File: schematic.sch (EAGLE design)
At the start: 25 parts

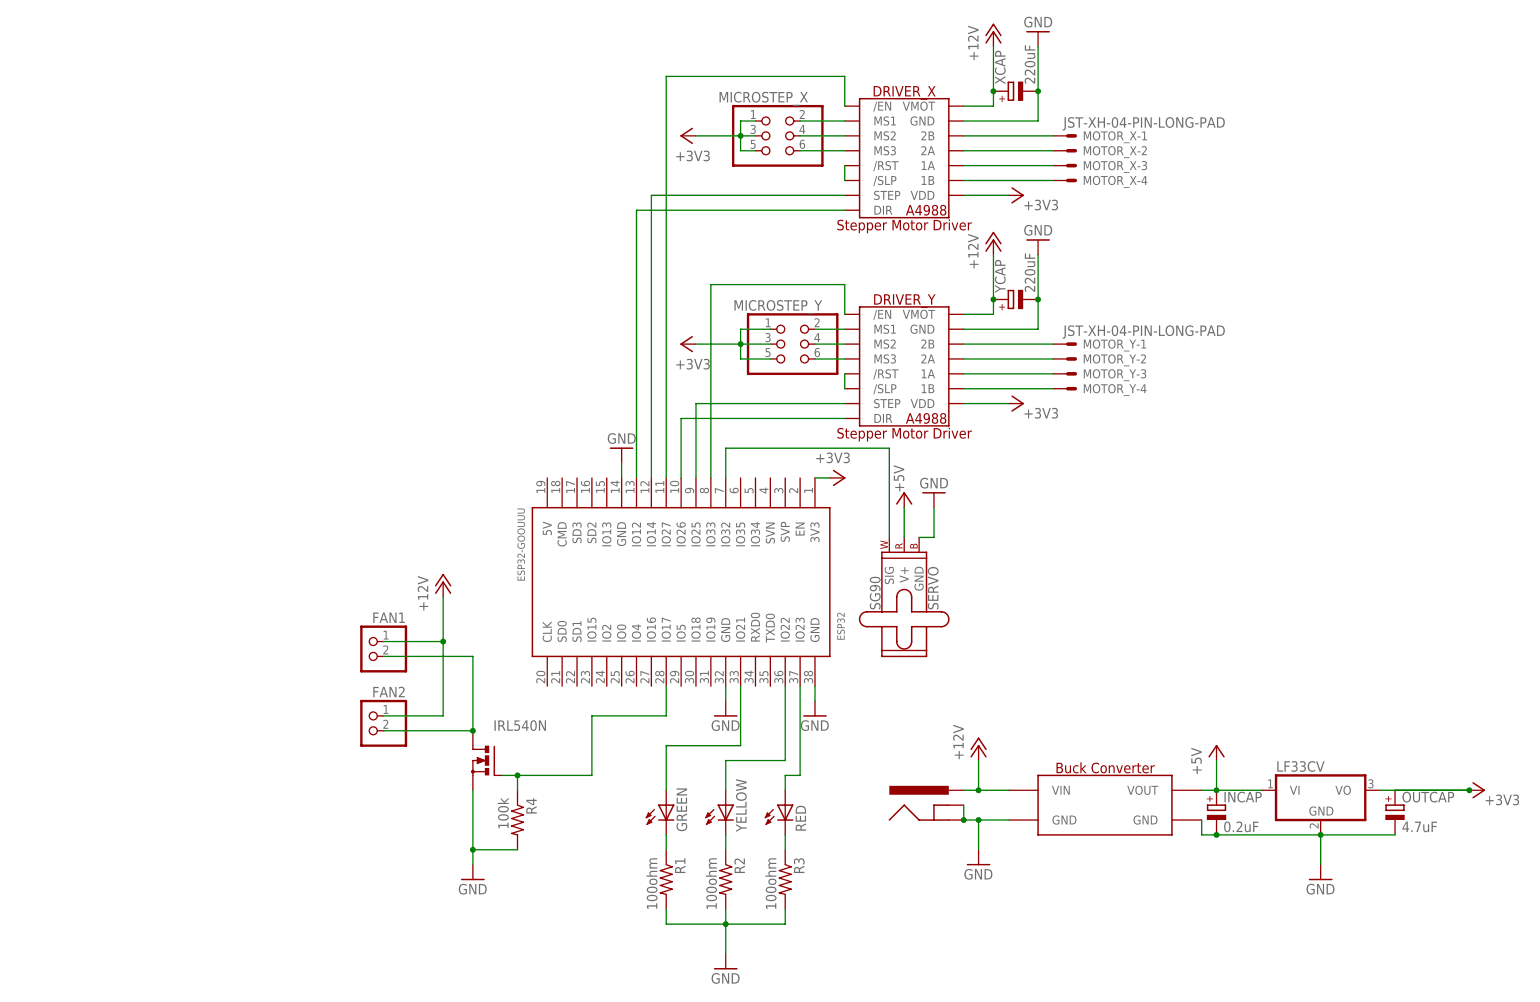
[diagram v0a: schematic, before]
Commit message: akjdf;sjf
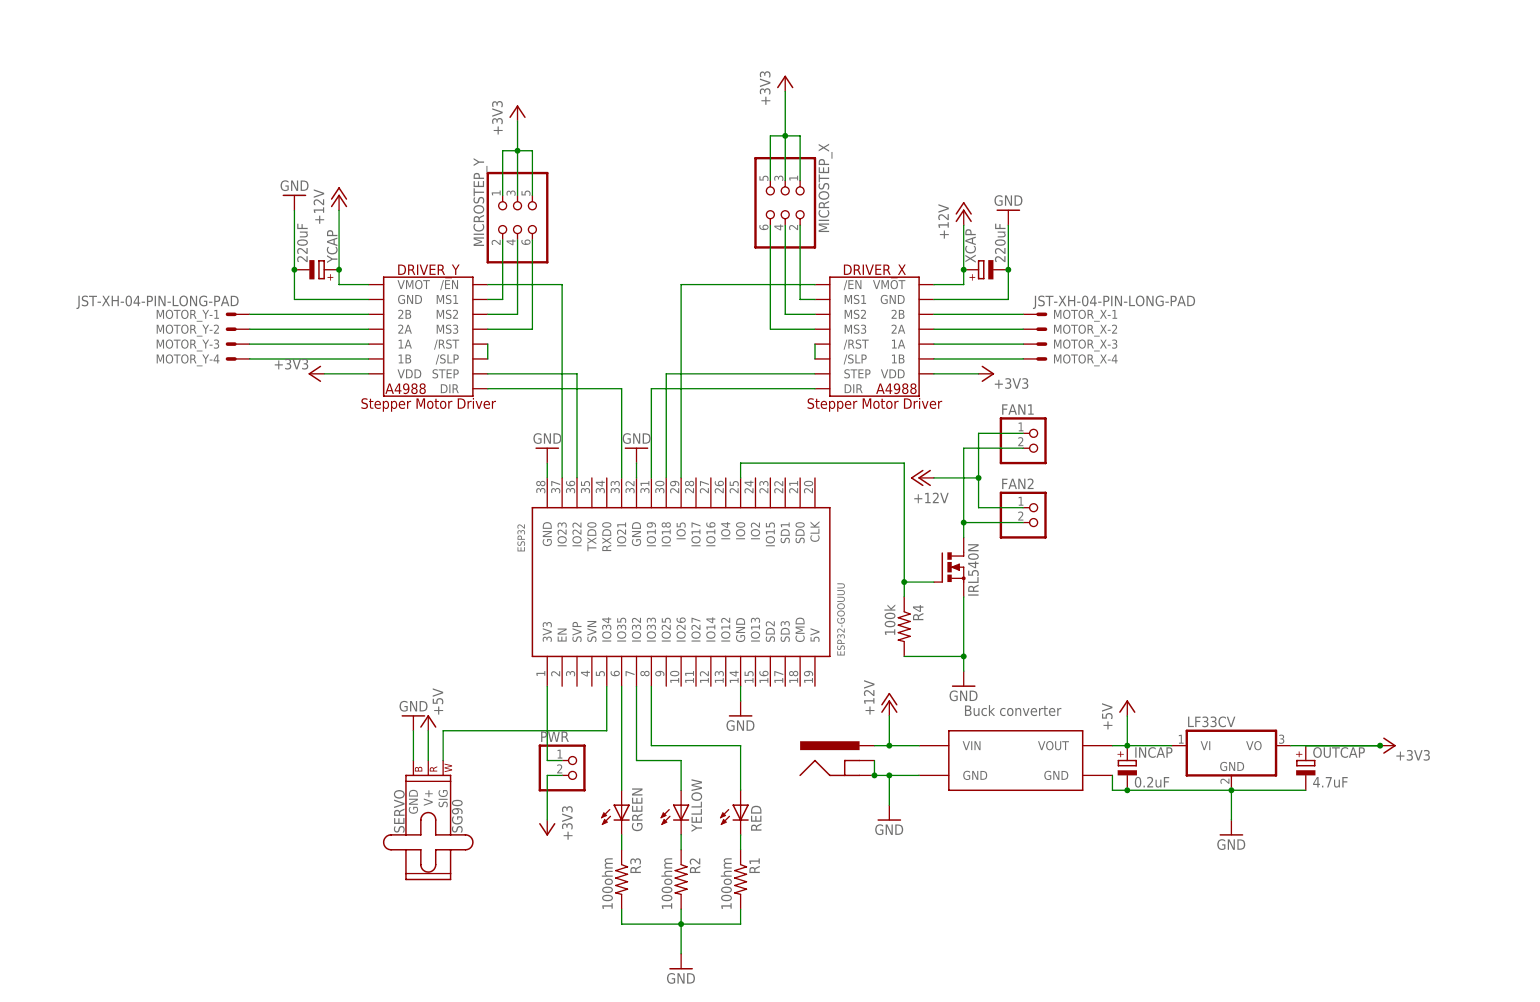
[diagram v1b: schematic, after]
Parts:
- removed U$1: BUCK-CONVERTER, buck-converter:BUCK-CONVERTER
- added PWR: (no value), pinhead:PINHD-1X2
- added U$2: BUCK-CONVERTER, mine:BUCK-CONVERTER
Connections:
- net MS1_X renamed N$11
- net MS1_Y renamed N$5
- net MS2_X renamed N$12
- net MS2_Y renamed N$9
- net MS3_X renamed N$13
- net MS3_Y renamed N$10
- net N$32 renamed FAN_PW
- removed net N$15: DRIVER_X./EN, ESP32.IO27
- removed net N$19: DRIVER_Y./EN, ESP32.IO33
- removed net N$2: DRIVER_X.STEP, ESP32.IO14
- removed net N$23: ESP32.IO23, RED.A
- removed net N$25: GREEN.C, R1.1
- removed net N$26: ESP32.IO21, GREEN.A
- removed net N$27: ESP32.IO22, YELLOW.A
- removed net N$29: R3.1, RED.C
- removed net N$30: ESP32.IO32, SG90.SIG
- removed net N$31: ESP32.IO17, IRL540N.G, R4.1
- removed net N$4: DRIVER_Y.DIR, ESP32.IO26
- removed net N$5 (its old number): DRIVER_Y.STEP, ESP32.IO25
- new net FAN_EN: ESP32.IO0, IRL540N.G, R4.1
- new net GREEN_LED: ESP32.IO35, GREEN.A
- new net N$21: R1.1, RED.C
- new net N$8: GREEN.C, R3.1
- new net RED_LED: ESP32.IO33, RED.A
- new net SERVO: ESP32.IO34, SG90.SIG
- new net X_DIR: DRIVER_X.DIR, ESP32.IO19
- new net X_EN: DRIVER_X./EN, ESP32.IO5
- new net X_STEP: DRIVER_X.STEP, ESP32.IO18
- new net YELLOW_LED: ESP32.IO32, YELLOW.A
- new net Y_DIR: DRIVER_Y.DIR, ESP32.IO21
- new net Y_EN: DRIVER_Y./EN, ESP32.IO23
- new net Y_STEP: DRIVER_Y.STEP, ESP32.IO22
- net +12V: now also U$2.VIN; no longer U$1.VIN
- net +3V3: now also PWR.2; no longer ESP32.3V3
- net +5V: now also U$2.VOUT; no longer U$1.VOUT
- net GND: now also U$2.GND@1, U$2.GND@2; no longer U$1.GND@1, U$1.GND@2
- net N$1: now also ESP32.3V3, PWR.1; no longer DRIVER_X.DIR, ESP32.IO12
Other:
- moved on the sheet: DRIVER_X, DRIVER_Y, ESP32, FAN1, FAN2, GREEN, INCAP, IRL540N, LF33CV, MICROSTEP_X, MICROSTEP_Y, MOTOR_X-1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
